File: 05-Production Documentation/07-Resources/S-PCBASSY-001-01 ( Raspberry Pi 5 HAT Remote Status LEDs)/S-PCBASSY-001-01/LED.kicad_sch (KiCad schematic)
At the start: 4 parts

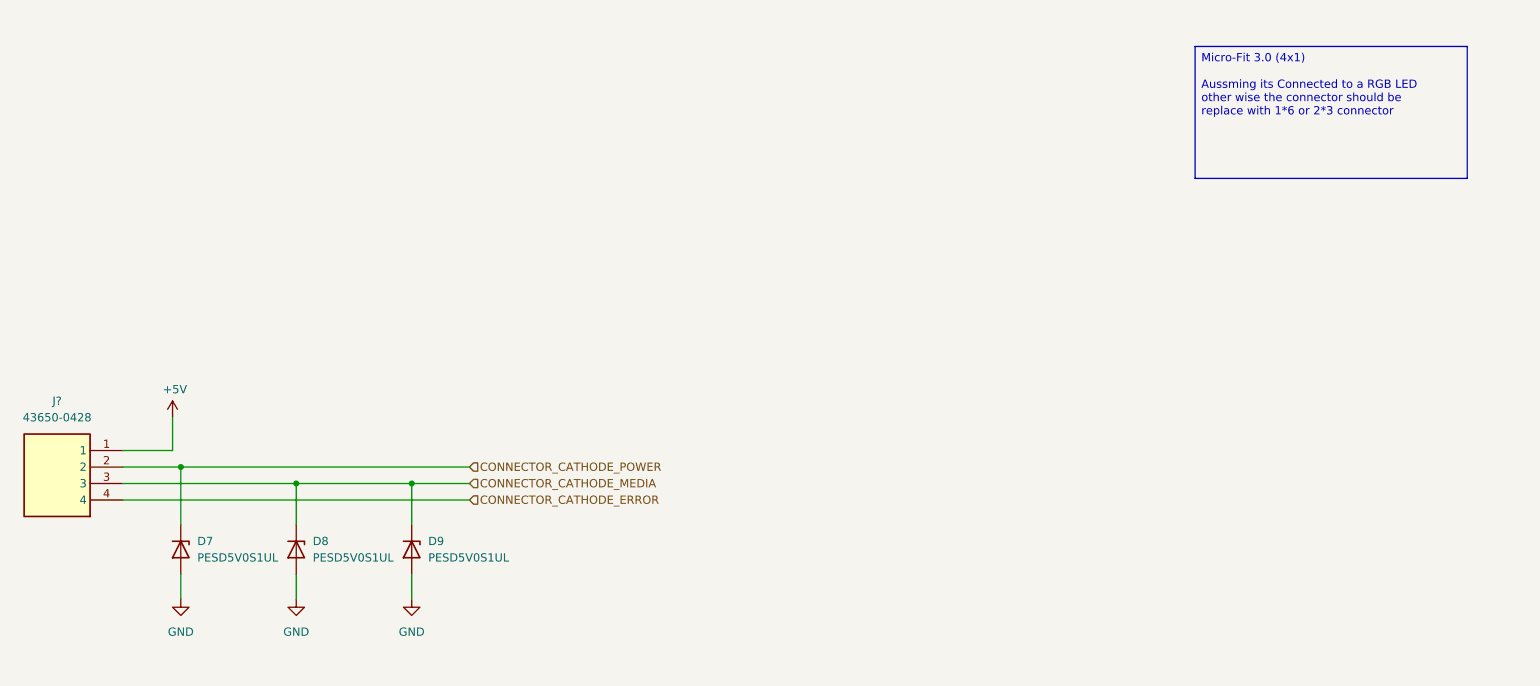
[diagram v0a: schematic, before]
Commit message: Schematics done
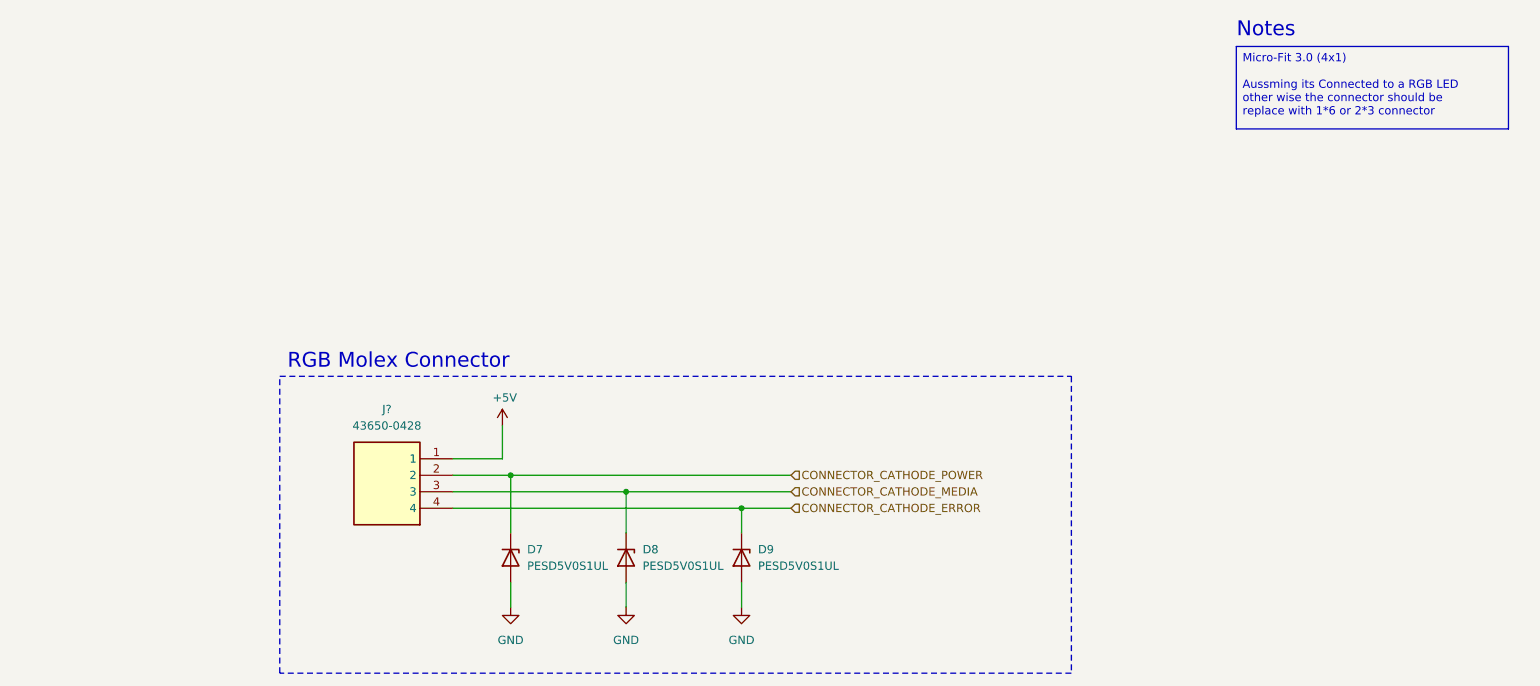
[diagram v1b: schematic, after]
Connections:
- net CONNECTOR_CATHODE_ERROR: now also D9.1 (K)
- net CONNECTOR_CATHODE_MEDIA: no longer D9.1 (K)
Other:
- note added: "Notes"
- note added: "RGB Molex Connector"
- moved on the sheet: D7, D8, D9, J?
